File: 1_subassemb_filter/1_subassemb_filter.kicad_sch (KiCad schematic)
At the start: 9 parts

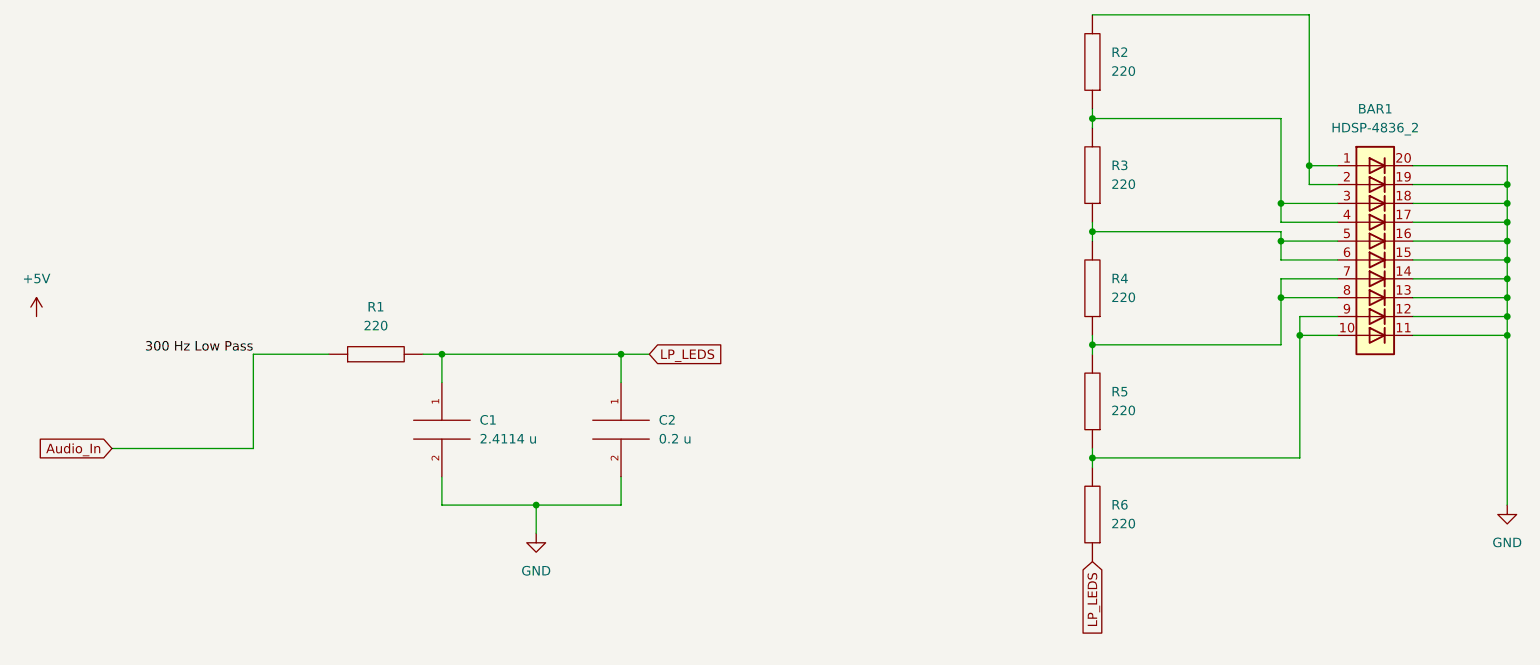
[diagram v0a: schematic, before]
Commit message: Updates to the filter
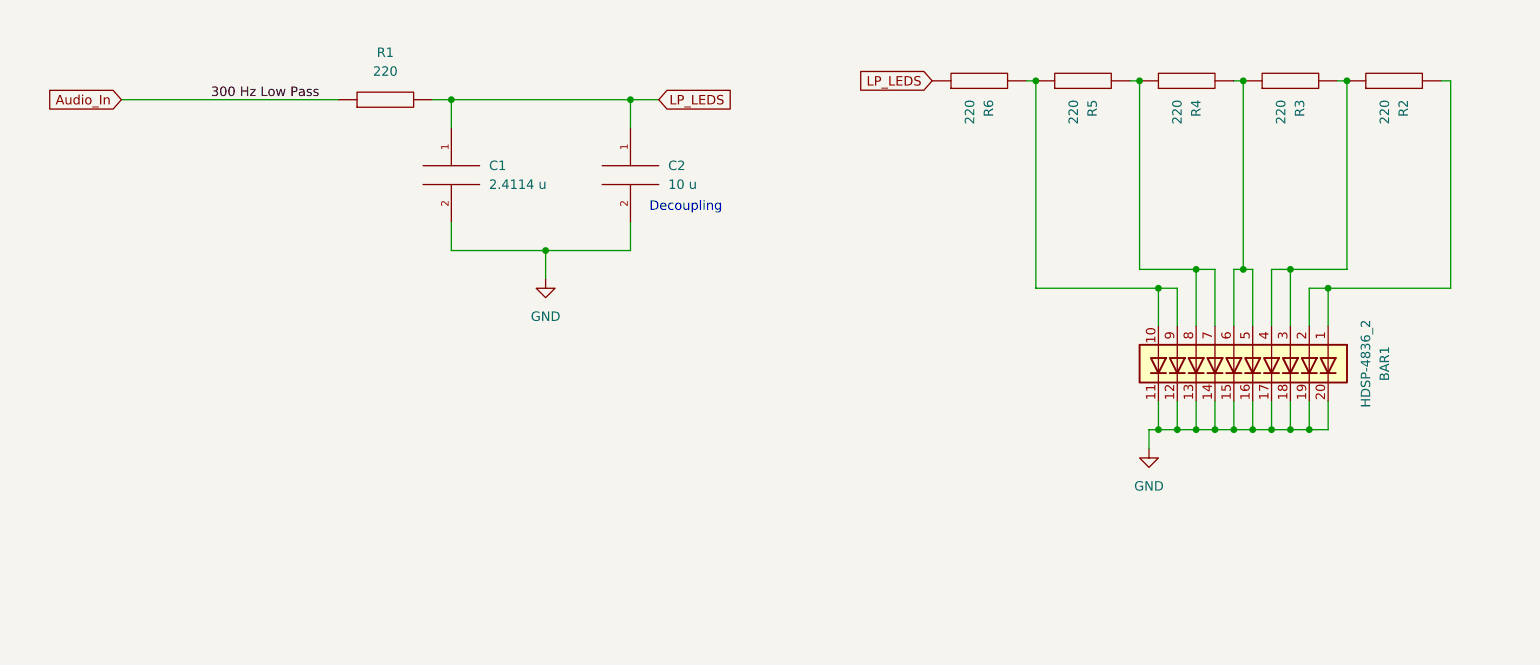
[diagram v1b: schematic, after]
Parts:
- C2: value 0.2 u -> 10 u
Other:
- note added: "Decoupling"
- moved on the sheet: BAR1, C1, C2, R1, R2, R3, R4, R5, R6
